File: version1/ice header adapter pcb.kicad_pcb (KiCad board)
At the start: 2 copper layers, 37.1 x 48.3 mm, 10 parts, among them P1 TST, P2 TST, P3 TST, P4 TST

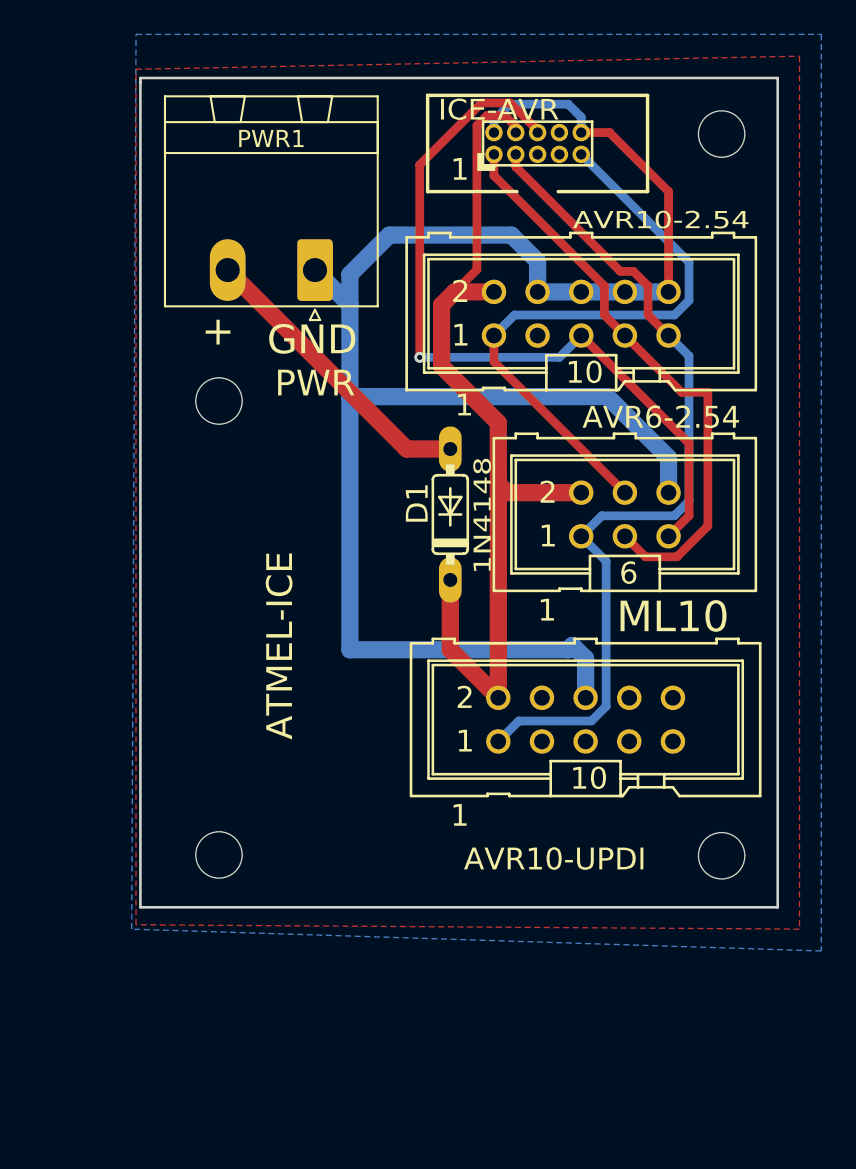
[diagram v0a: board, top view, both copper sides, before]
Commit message: weiter am pc
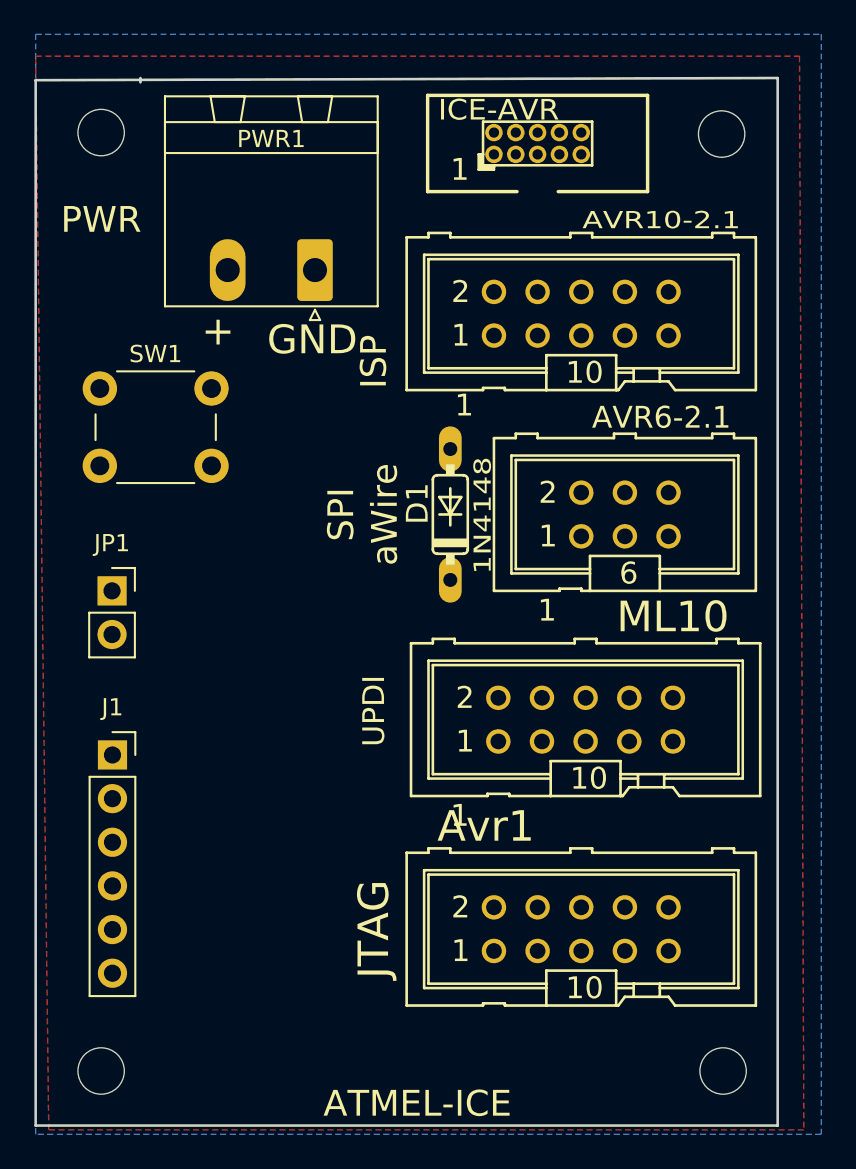
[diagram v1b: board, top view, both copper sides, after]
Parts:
- added Avr1: JTAG, con-harting-ml:ML10, F.Cu at (87.6, 161.3)
- added J1: FTDI 232, Connector_PinSocket_2.54mm:PinSocket_1x06_P2.54mm_Vertical, F.Cu at (60.4, 151.2)
- added JP1: FTDI_VCC, Connector_PinSocket_2.54mm:PinSocket_1x02_P2.54mm_Vertical, F.Cu at (60.3, 141.6)
- added SW1: Reset, Button_Switch_THT:SW_PUSH_6mm_H5mm, F.Cu at (59.6, 129.8)
- moved P1 17.1 mm to (59.7, 114.9)
- moved P3 14.3 mm to (59.7, 169.5)
- moved P4 12.5 mm to (95.9, 169.5)
- renumbered AVR10-2.54 to AVR10-2.1, AVR6-2.54 to AVR6-2.1, AVR10-UPDI to UPDI
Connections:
- UPDI pad 3: unconnected-(AVR10-UPDI1-Pad3) -> /RX
- UPDI pad 4: unconnected-(AVR10-UPDI1-Pad4) -> /TX
- UPDI pad 5: unconnected-(AVR10-UPDI1-Pad5) -> /RESET
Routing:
- net /GND: track 104.8 -> 0.00 mm
- net /VTG: track 55.1 -> 0.00 mm
- net /TDO: track 49.5 -> 0.00 mm
- net /NSRST: track 45.0 -> 0.00 mm, vias 1 -> 0
- net /TDI: track 35.6 -> 0.00 mm
- net /TCK: track 33.7 -> 0.00 mm
- net Net-(D1-PadA): track 17.3 -> 0.00 mm
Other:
- board size 37.1 x 48.3 mm -> 43.2 x 61 mm
- board text added: "ISP"
- board text added: "SPI"
- board text added: "aWire"
